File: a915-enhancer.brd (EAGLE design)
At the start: 100 x 50 mm, 74 parts, among them U1 SCREW-M2X8, U10 FX2-20S-1.27DS, U2 SCREW-M2X8, U3 NUT-M2-SELFLOCK, U4 NUT-M2-SELFLOCK, U5 FX2-20P-1.27DS, U6 SCREW-M2X8, U7 SCREW-M2X8, U8 NUT-M2-SELFLOCK, U9 NUT-M2-SELFLOCK

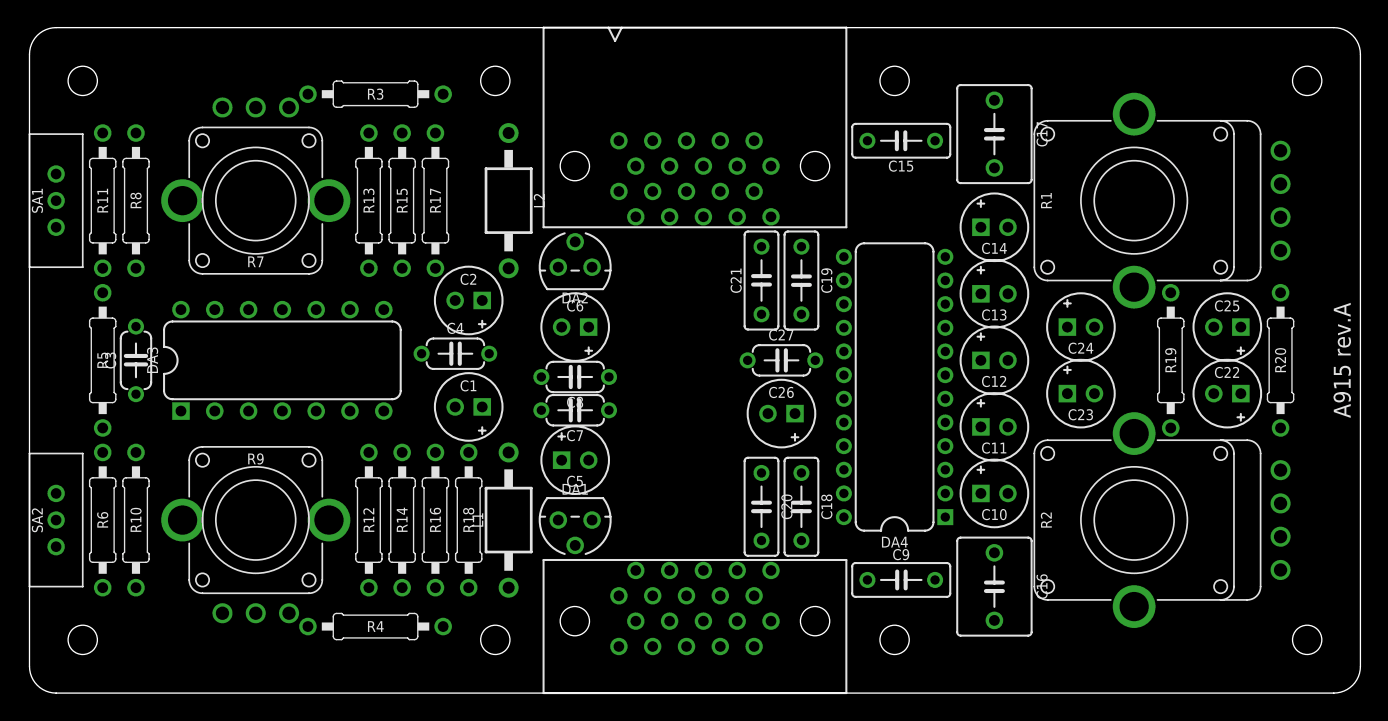
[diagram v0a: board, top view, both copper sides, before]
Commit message: A915a Routing
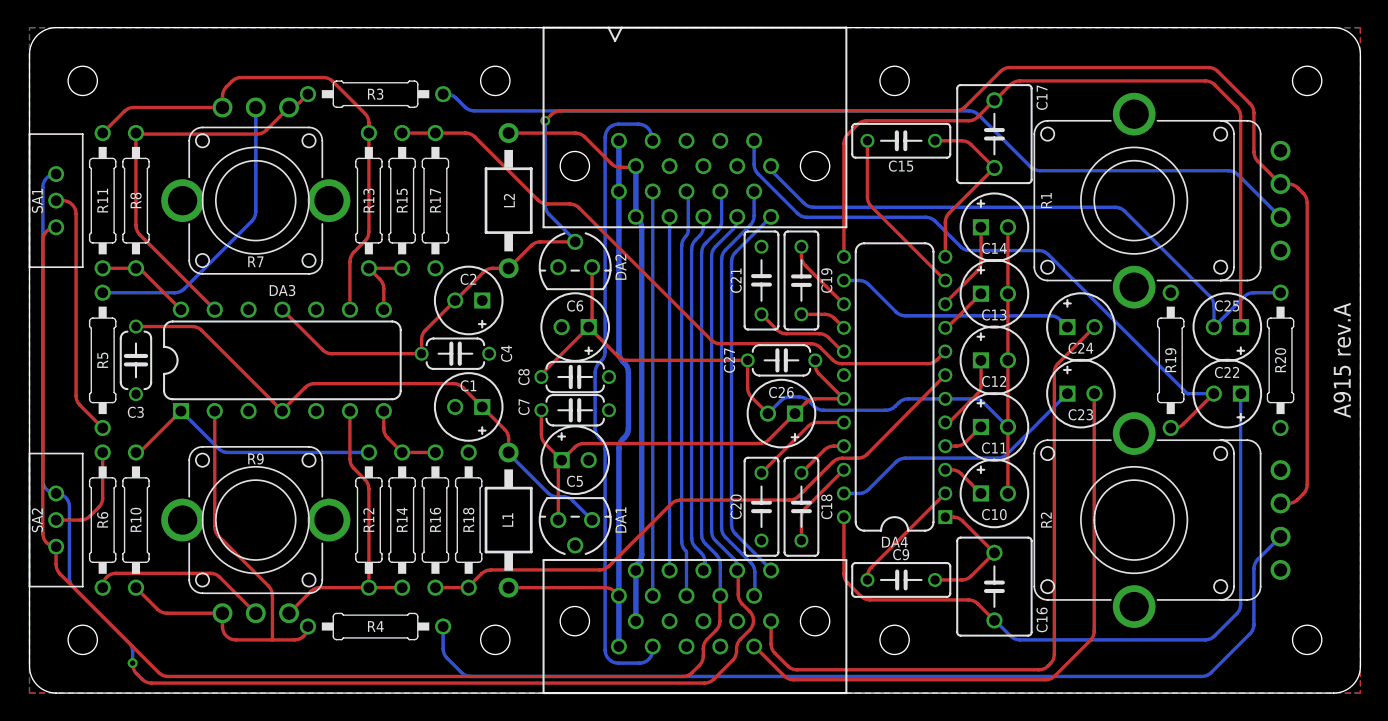
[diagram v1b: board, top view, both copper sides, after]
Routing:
- net -15V: track 0.00 -> 126.4 mm, vias 0 -> 1
- net CV2: track 0.00 -> 121.8 mm, vias 0 -> 1
- net CV1: track 0.00 -> 115.4 mm
- net N$39: track 0.00 -> 72.7 mm
- net -5V: track 0.00 -> 67.0 mm
- net N$10: track 0.00 -> 66.4 mm
- net N$33: track 0.00 -> 57.3 mm
- net N$32: track 0.00 -> 53.2 mm
- net N$42: track 0.00 -> 50.3 mm
- net N$16: track 0.00 -> 48.1 mm
- net DEFINITION: track 0.00 -> 47.9 mm
- net N$41: track 0.00 -> 47.6 mm
- net N$1: track 0.00 -> 46.8 mm
- net N$40: track 0.00 -> 46.0 mm
- net N$44: track 0.00 -> 45.4 mm
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- added copper zone on layer 1, net GND
- added copper zone on layer 16, net GND
